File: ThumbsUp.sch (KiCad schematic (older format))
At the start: 150 parts, among them IC1 RP2040, IC2 W25Q128JVSIM, J1 Conn_01x04_Male, J10 Raiser_Male, J11 Raiser_Female, J12 Raiser_Male, J13 Raiser_Female, J14 Raiser_Male, J15 Raiser_Female, J16 Raiser_Male, J17 Raiser_Female, J18 Raiser_Male, J19 52559-1233, J2 Conn_01x04_Male, J20 Conn_01x04_Female, J21 Conn_01x04_Female, J22 Conn_01x04_Female, J23 Conn_01x04_Female, J24 Conn_01x04_Male, J25 Conn_01x04_Male, J26 Conn_01x04_Male, J27 Conn_01x04_Male, J28 Conn_01x04_Female, J29 Conn_01x04_Female, J3 Conn_01x04_Female, J30 Conn_01x04_Female, J31 Conn_01x04_Female, J4 Conn_01x04_Male, J5 Conn_01x04_Female, J6 Conn_01x04_Male, J7 Conn_01x04_Male, J8 Conn_01x04_Male, J9 Raiser_Female, U1 NCP1117-3.3_SOT223, Y1 ABLS-12.000MHZ-B4-T

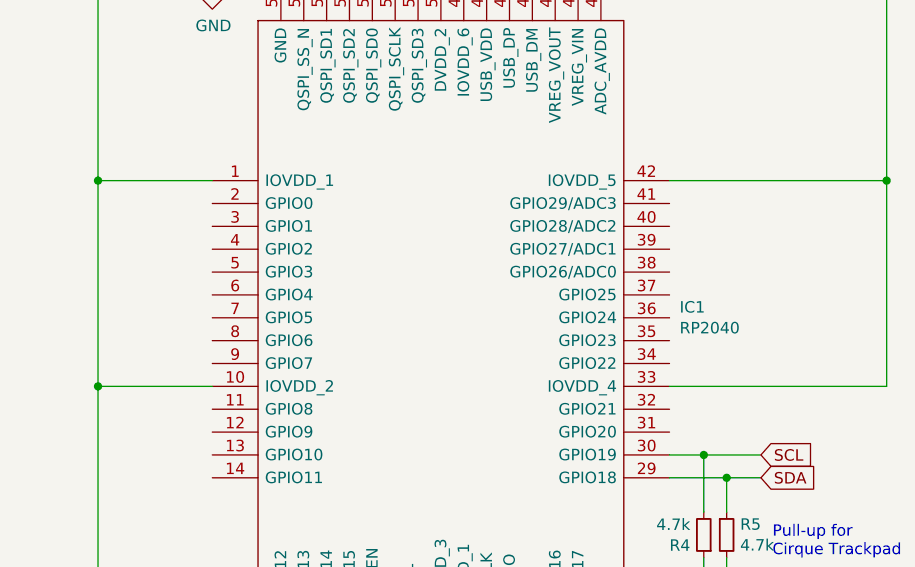
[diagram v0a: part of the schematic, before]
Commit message: Wiring continued
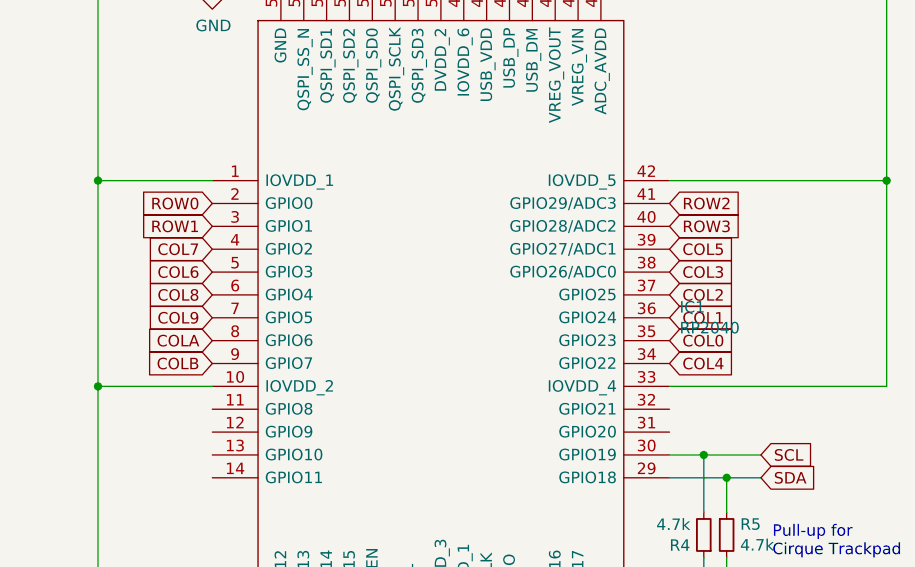
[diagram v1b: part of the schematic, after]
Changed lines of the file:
@@
 Wire Wire Line
 	12550 2900 12200 2900
-$Comp
-L RP2040:RP2040 IC1
-U 1 1 6393717F
-P 2050 2550
-F 0 "IC1" H 4094 1996 50  0000 L CNN
-F 1 "RP2040" H 4094 1905 50  0000 L CNN
-F 2 "RP2040:QFN40P700X700X90-57N-D" H 3900 3250 50  0001 L CNN
-F 3 "https://datasheets.raspberrypi.org/rp2040/rp2040-datasheet.pdf" H 3900 3150 50  0001 L CNN
-F 4 "Microcontroller in QFN Package" H 3900 3050 50  0001 L CNN "Description"
-F 5 "0.9" H 3900 2950 50  0001 L CNN "Height"
-F 6 "RASPBERRY-PI" H 3900 2850 50  0001 L CNN "Manufacturer_Name"
-F 7 "RP2040" H 3900 2750 50  0001 L CNN "Manufacturer_Part_Number"
-F 8 "" H 3900 2650 50  0001 L CNN "Mouser Part Number"
-F 9 "" H 3900 2550 50  0001 L CNN "Mouser Price/Stock"
-F 10 "" H 3900 2450 50  0001 L CNN "Arrow Part Number"
-F 11 "" H 3900 2350 50  0001 L CNN "Arrow Price/Stock"
-F 12 "" H 3900 2250 50  0001 L CNN "Mouser Testing Part Number"
-F 13 "" H 3900 2150 50  0001 L CNN "Mouser Testing Price/Stock"
-	1    2050 2550
-	1    0    0    -1
-$EndComp
 Wire Wire Line
 	2050 3450 1550 3450
@@
 Wire Wire Line
 	3050 5100 1550 5100
-Wire Wire Line
-	1550 5100 1550 3450
 Connection ~ 1550 3450
 Wire Wire Line
@@
 Wire Wire Line
 	1550 1200 1550 2550
-Wire Wire Line
-	2050 2550 1550 2550
 Connection ~ 1550 2550
 Wire Wire Line
@@
 	3550 5050 3550 5350
 Connection ~ 3550 5350
+Wire Wire Line
+	1550 5100 1550 3450
+Wire Wire Line
+	2050 2550 1550 2550
+$Comp
+L RP2040:RP2040 IC1
+U 1 1 6393717F
+P 2050 2550
+F 0 "IC1" H 4094 1996 50  0000 L CNN
+F 1 "RP2040" H 4094 1905 50  0000 L CNN
+F 2 "RP2040:QFN40P700X700X90-57N-D" H 3900 3250 50  0001 L CNN
+F 3 "https://datasheets.raspberrypi.org/rp2040/rp2040-datasheet.pdf" H 3900 3150 50  0001 L CNN
+F 4 "Microcontroller in QFN Package" H 3900 3050 50  0001 L CNN "Description"
+F 5 "0.9" H 3900 2950 50  0001 L CNN "Height"
+F 6 "RASPBERRY-PI" H 3900 2850 50  0001 L CNN "Manufacturer_Name"
+F 7 "RP2040" H 3900 2750 50  0001 L CNN "Manufacturer_Part_Number"
+F 8 "" H 3900 2650 50  0001 L CNN "Mouser Part Number"
+F 9 "" H 3900 2550 50  0001 L CNN "Mouser Price/Stock"
+F 10 "" H 3900 2450 50  0001 L CNN "Arrow Part Number"
+F 11 "" H 3900 2350 50  0001 L CNN "Arrow Price/Stock"
+F 12 "" H 3900 2250 50  0001 L CNN "Mouser Testing Part Number"
+F 13 "" H 3900 2150 50  0001 L CNN "Mouser Testing Price/Stock"
+	1    2050 2550
+	1    0    0    -1
+$EndComp
+Text GLabel 4050 2650 2    50   Input ~ 0
+ROW2
+Text GLabel 4050 2750 2    50   Input ~ 0
+ROW3
+Text GLabel 4050 2850 2    50   Input ~ 0
+COL5
+Text GLabel 4050 2950 2    50   Input ~ 0
+COL3
+Text GLabel 4050 3050 2    50   Input ~ 0
+COL2
+Text GLabel 4050 3150 2    50   Input ~ 0
+COL1
+Text GLabel 4050 3250 2    50   Input ~ 0
+COL0
+Text GLabel 4050 3350 2    50   Input ~ 0
+COL4
+Text GLabel 2050 2650 0    50   Input ~ 0
+ROW0
+Text GLabel 2050 2750 0    50   Input ~ 0
+ROW1
+Text GLabel 2050 2850 0    50   Input ~ 0
+COL7
+Text GLabel 2050 2950 0    50   Input ~ 0
+COL6
+Text GLabel 2050 3050 0    50   Input ~ 0
+COL8
+Text GLabel 2050 3150 0    50   Input ~ 0
+COL9
+Text GLabel 2050 3250 0    50   Input ~ 0
+COLA
+Text GLabel 2050 3350 0    50   Input ~ 0
+COLB
 $EndSCHEMATC
